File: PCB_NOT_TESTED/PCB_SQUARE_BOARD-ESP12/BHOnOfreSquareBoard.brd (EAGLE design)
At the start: 47.6 x 47.7 mm, 23 parts, among them J1 4p, J6 8p, J7 8p, K1 OMRON-G3MB-202P-SSR2, K2 OMRON-G3MB-202P-SSR2, Q1 S8050, Q2 S8050, U1 LM1117, U2 esp12

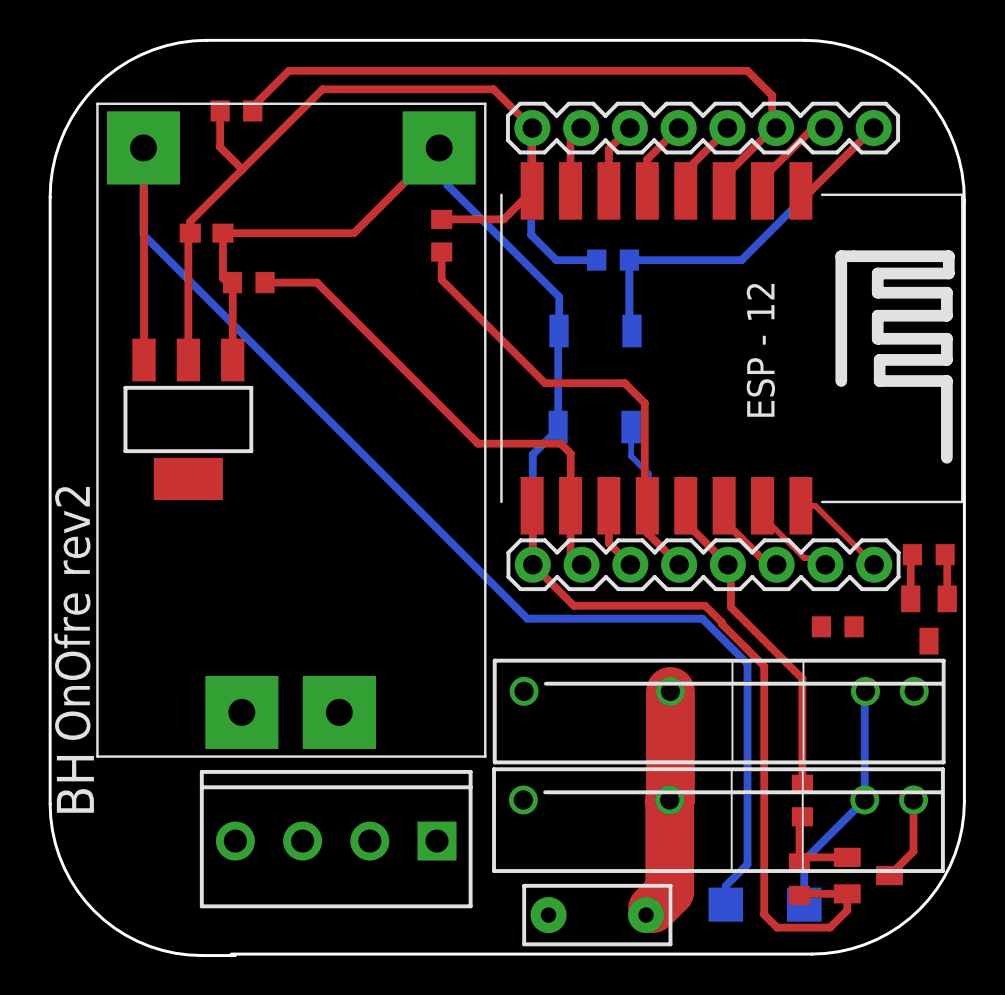
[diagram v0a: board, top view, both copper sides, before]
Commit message: Square Rev2 pronto para testes
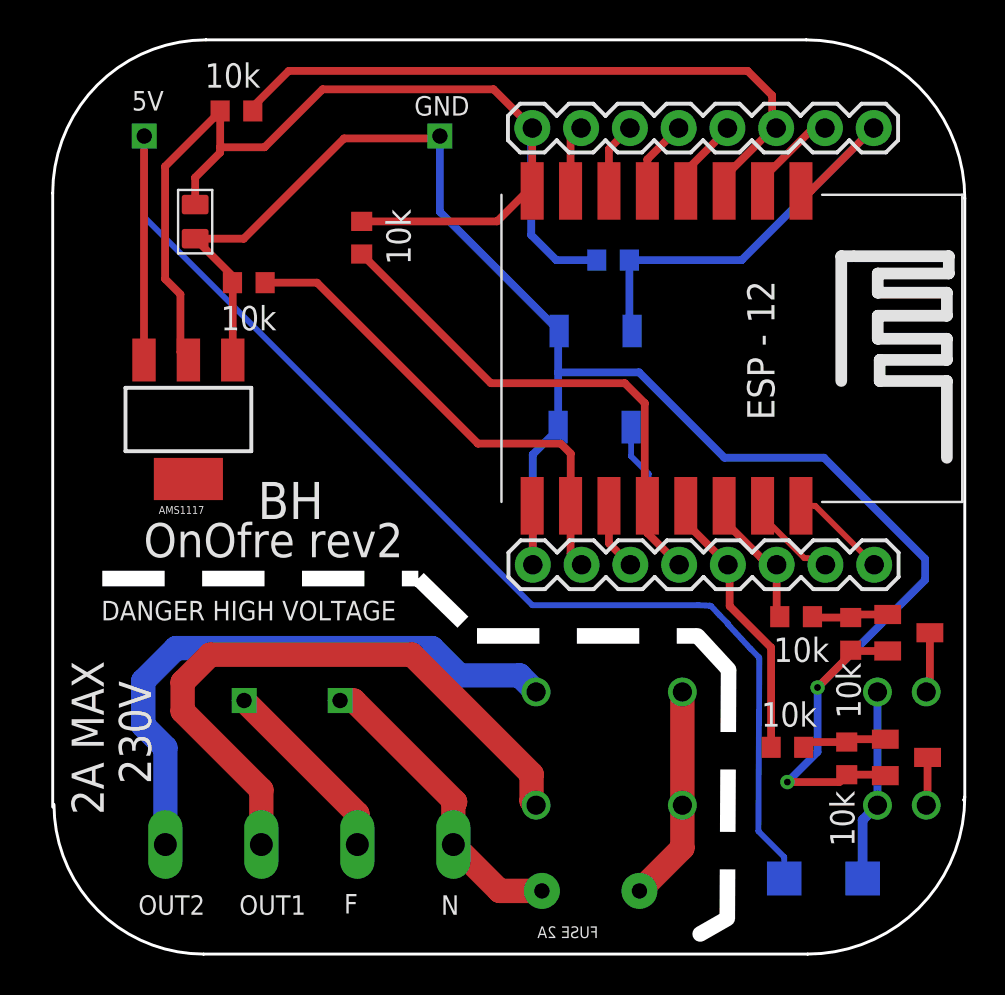
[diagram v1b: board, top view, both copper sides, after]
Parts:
- removed J1: 4p, SparkFun-Connectors:SCREWTERMINAL-3.5MM-4
- removed Q2: S8050, semicon-smd-ipc:SOT23
- added JY3: S8050, semicon-smd-ipc:SOT23
- added X2: PLUG, con-wago-500:W237-4
- C4: value 100nF -> 100nf; device SparkFun-Capacitors:0603 -> Seeed-Capacitor:C0805
- U$2: value HLK-PM03 -> HKLPM01; device PowerSocket:HLK-PM03 -> HKLPM01:HKLPM01
- moved U$2 15.5 mm to (12.6, 27.9), flipped to the bottom
- moved R3 6.76 mm to (41.5, 10.2)
- moved Q1 6.47 mm to (44.6, 10.2)
- moved R2 5.80 mm to (41.7, 16.7), turned to 90 degrees
- moved R8 4.17 mm to (16.2, 37.3)
- moved D3 3.33 mm to (40.3, 3.94)
- moved R4 2.88 mm to (38.4, 10.8), turned to 0 degrees
- moved R1 2.23 mm to (38.9, 17.6)
- moved F1 1.31 mm to (28.2, 3.29), flipped to the bottom, turned to 180 degrees
- moved C4 0.85 mm to (7.55, 38.1)
- moved K1 0.71 mm to (38.0, 7.75), flipped to the bottom, turned to 180 degrees
- moved K2 0.62 mm to (38.0, 13.7), flipped to the bottom, turned to 180 degrees
- renumbered U1 to AMS1117
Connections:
- removed net FASE: J1.3, U$2.AC2
- new net FASE_IN: U$2.P$2, X2.2
- net GND: now also JY3.2, U$2.P$3; no longer Q2.2, U$2.-VO
- net N$13: now also JY3.1; no longer Q2.1
- net N$9: now also JY3.3; no longer Q2.3
- net NEUTRAL_IN: now also U$2.P$1, X2.1; no longer J1.4, U$2.AC1
- net NEUTRAL_ONE_OUT: now also X2.3; no longer J1.2
- net NEUTRAL_TWO_OUT: now also X2.4; no longer J1.1
- net VCC: now also U$2.P$4; no longer U$2.+VO
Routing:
- net NEUTRAL_ONE_OUT: track 0.00 -> 33.2 mm
- net NEUTRAL_TWO_OUT: track 0.00 -> 31.1 mm
- net NEUTRAL_IN: track 0.00 -> 16.1 mm
- net GND: track 86.1 -> 98.4 mm, vias 0 -> 2
- net 3V3: track 51.3 -> 61.8 mm
- net FASE_IN: track 0.00 -> 9.94 mm
- net GPIO0: track 32.5 -> 35.7 mm
- net N$9: track 0.00 -> 3.16 mm
- net GPIO04: track 4.47 -> 7.24 mm
- net GPIO05: track 17.2 -> 14.5 mm
- net N$2: track 12.4 -> 10.0 mm
- net N$1: track 4.46 -> 2.52 mm
- net N$13: track 2.35 -> 4.00 mm
- net N$7: track 5.07 -> 4.42 mm
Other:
- board size 47.6 x 47.7 mm -> 47.5 x 47.6 mm
- board text added: "00"
- board text added: "02"
- board text added: "04"
- board text added: "05"
- board text added: "12"
- board text added: "13"
- board text added: "14"
- board text added: "15"
- board text added: "16"
- board text added: "230V"
- board text added: "2A MAX"
- board text added: "3V3"
- board text added: "5V"
- board text added: "ADC"
- board text added: "DANGER HIGH VOLTAGE"
- board text added: "EN"
- board text added: "F"
- board text added: "FUSE 2A"
- board text added: "GND"
- board text added: "N"
- board text added: "OUT1"
- board text added: "OUT2"
- board text added: "RST"
- board text added: "RX"
- board text added: "TX"
- board text added: "www.movimentomaker.pt"
